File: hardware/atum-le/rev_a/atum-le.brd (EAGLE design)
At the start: 18.8 x 19.6 mm, 40 parts, among them J1 TC2030-JLINK-NL, J2 SH_MALE_2/1MM, J3 ATUM-HEADER, U2 FM25LBTDFN-8, U3 RV-3049-C3, U4 TPS62740, U5 NRF51822QF, X1 EPSON-FA-128, X2 ABS05-32.768KHZ-T

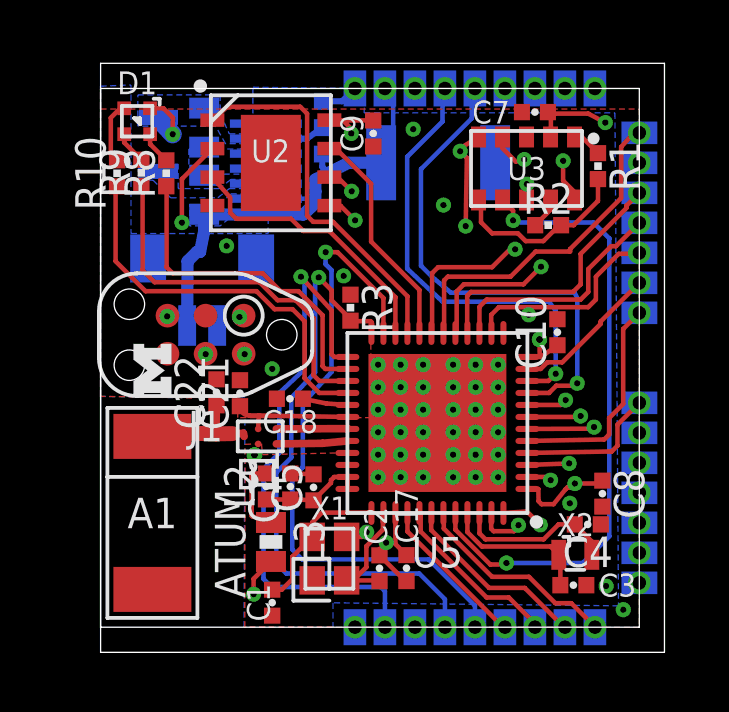
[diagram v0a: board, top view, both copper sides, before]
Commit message: fixed all drc errors
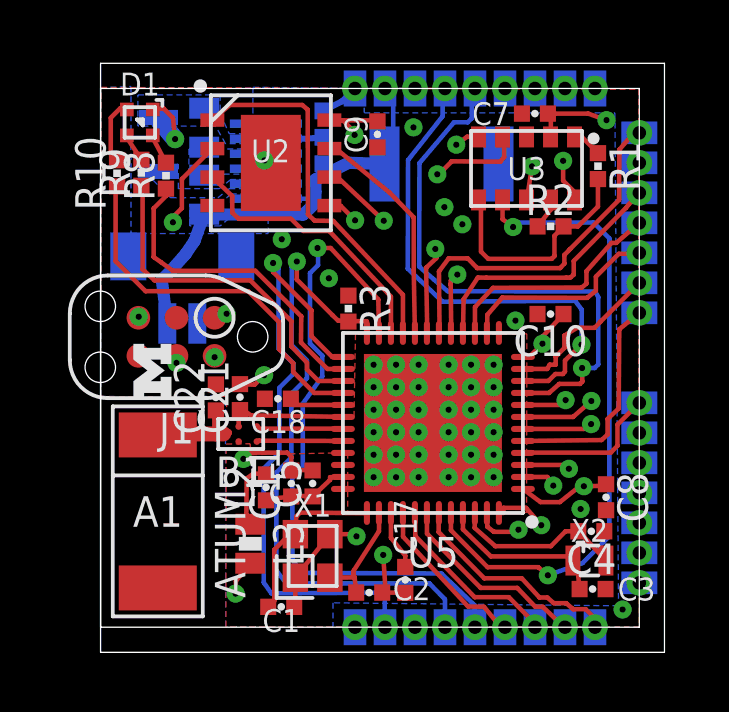
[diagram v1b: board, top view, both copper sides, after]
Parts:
- moved J1 0.97 mm to (2.53, 9.68)
- moved C2 0.88 mm to (8.95, 1.15), turned to 0 degrees
- moved L3 0.69 mm to (4.99, 2.78)
- moved J2 0.66 mm to (2.72, 10.0)
- moved B1 0.65 mm to (4.67, 6.44)
- moved C3 0.65 mm to (16.4, 1.27)
- moved C10 0.65 mm to (15.0, 10.4), turned to 180 degrees
- moved X1 0.57 mm to (7.07, 2.38)
- moved X2 0.51 mm to (16.3, 2.22)
- moved C18 0.40 mm to (5.91, 7.62)
- moved C17 0.39 mm to (10.2, 1.58)
- moved C1 0.33 mm to (6.02, 0.68), turned to 0 degrees
- moved U$1 0.32 mm to (7.41, 16.3)
- moved C4 0.26 mm to (16.4, 3.20)
- moved A1 0.19 mm to (1.91, 3.86)
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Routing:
- net GND: track 13.8 -> 22.0 mm, vias 50 -> 49
- net SPI_MISO: track 33.4 -> 36.8 mm
- net SWDCLK: track 25.9 -> 29.0 mm
- net AIN6: track 17.0 -> 18.7 mm
- net SPI_SCK: track 28.2 -> 26.5 mm
- net AIN7: track 15.2 -> 16.7 mm
- net SPI_MOSI: track 29.8 -> 31.1 mm
- net P17: track 19.7 -> 20.9 mm
- net SWDIO/!RESET: track 28.1 -> 29.1 mm
- net N$9: track 5.10 -> 6.06 mm
- net VCC: track 13.5 -> 14.4 mm, vias 7 -> 6
- net ANTENNA: track 4.10 -> 3.26 mm
- net N$18: track 2.40 -> 3.23 mm
- net N$6: track 5.03 -> 5.81 mm
- net BOOTLOADER_TX: track 11.4 -> 12.1 mm
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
